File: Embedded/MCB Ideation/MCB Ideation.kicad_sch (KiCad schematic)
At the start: 22 parts, among them J2 USB, J3 MicroSD, U1 ICM-20948, U2 BME280, U4 AP7366-33W5-7

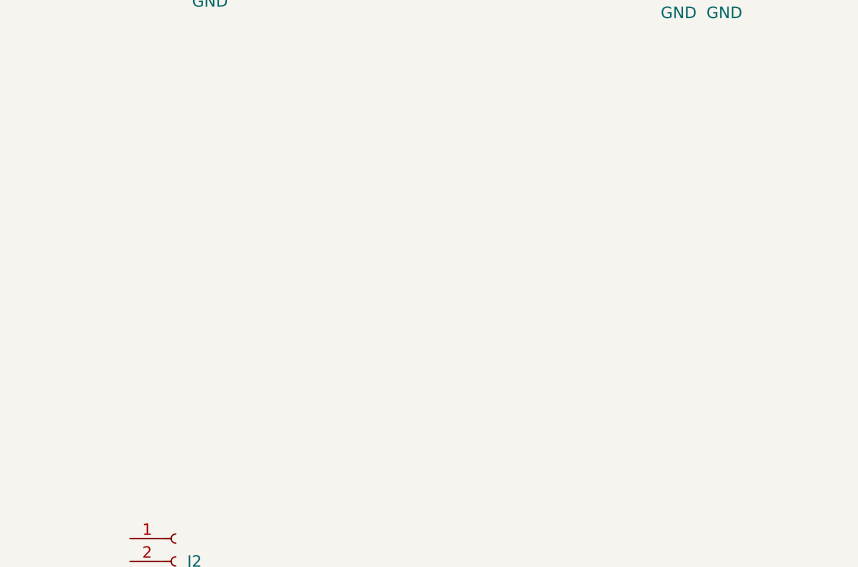
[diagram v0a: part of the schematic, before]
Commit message: Feature Listing & Organisation
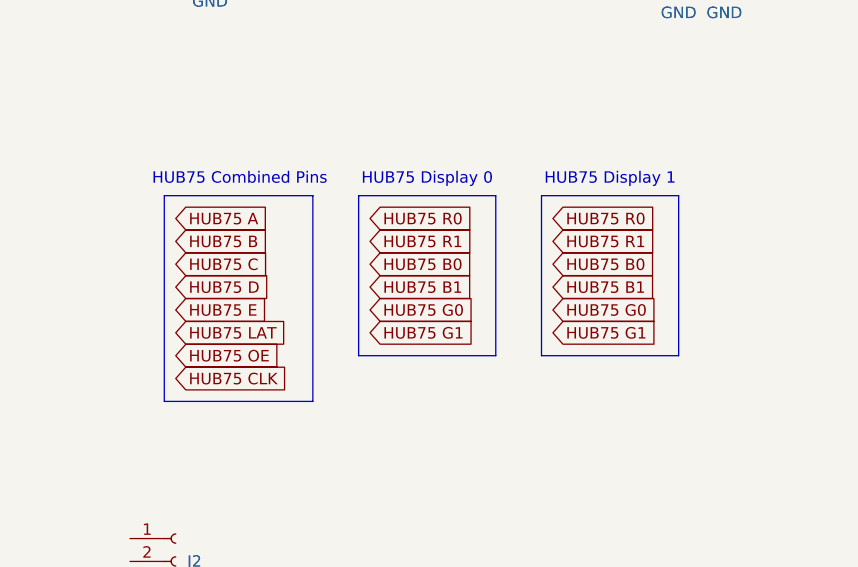
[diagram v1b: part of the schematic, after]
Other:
- note added: "HUB75 Combined Pins"
- note added: "HUB75 Display 0"
- note added: "HUB75 Display 1"
